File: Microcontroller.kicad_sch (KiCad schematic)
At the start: 33 parts, among them J501 USB4105-GF-A, J502 TC2030-CTX, SW501 PTS526SK15SMTR2 LFS, U501 USBLC6-2SC6, U502 STM32G441KBT6, Y501 ATS08A-E

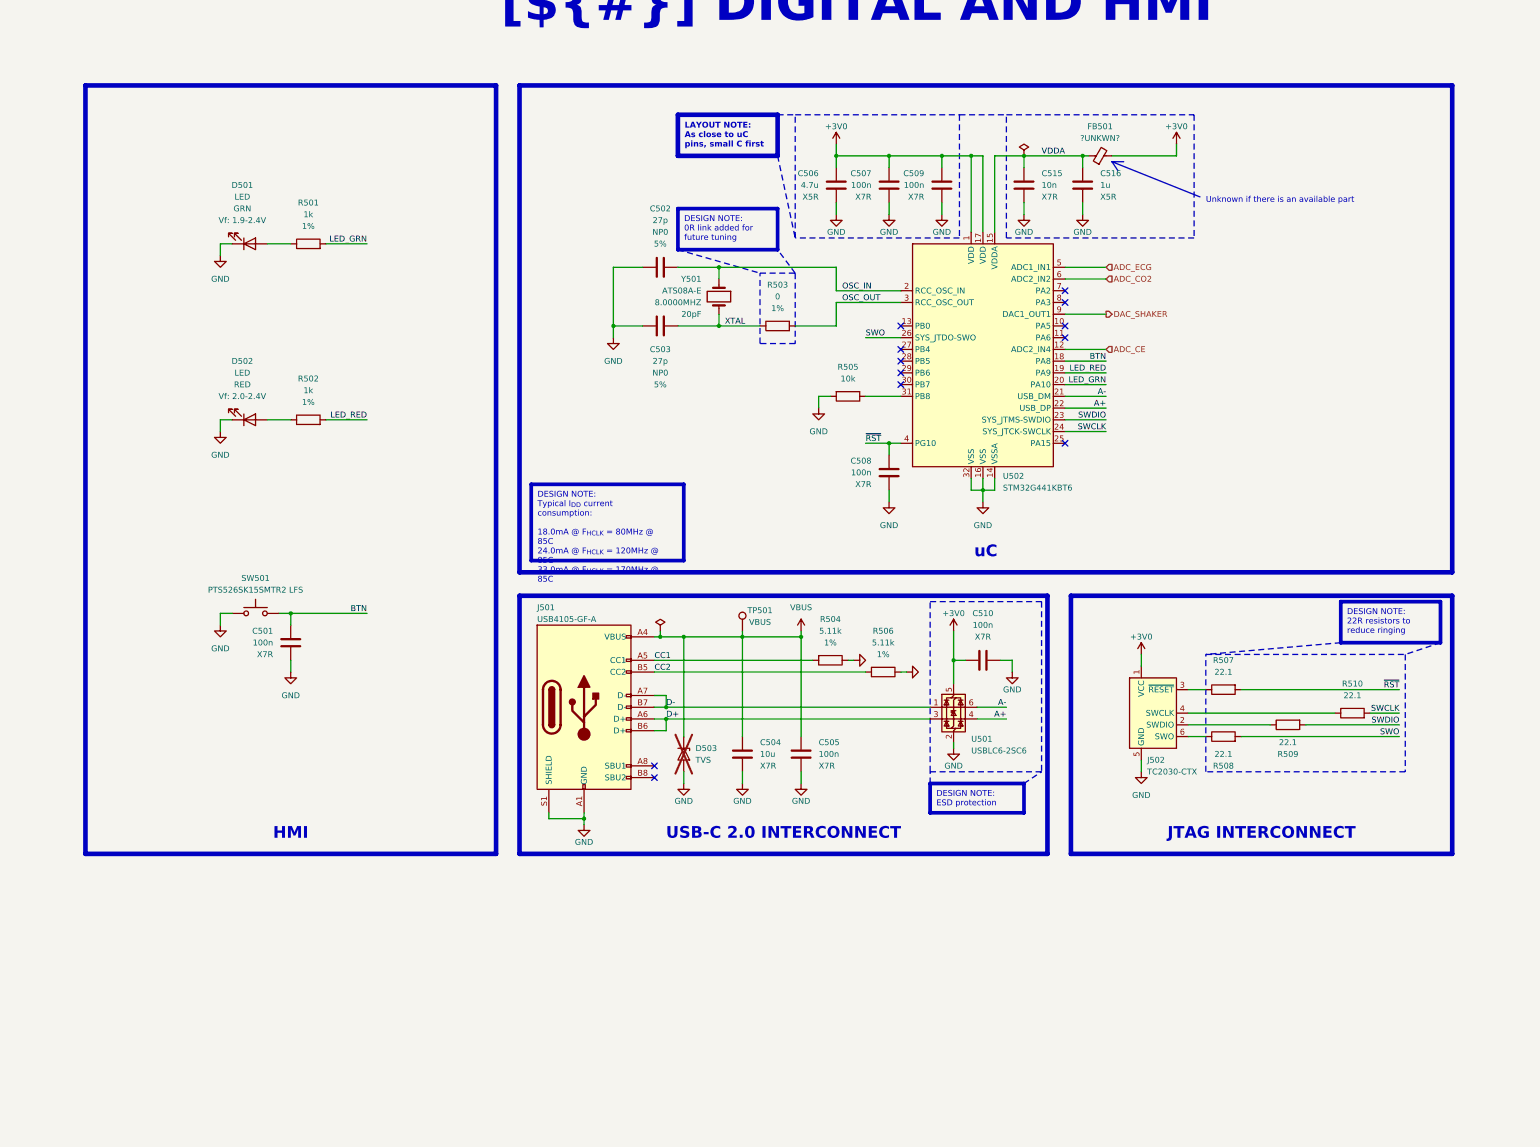
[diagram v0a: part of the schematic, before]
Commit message: feat: checked REV A
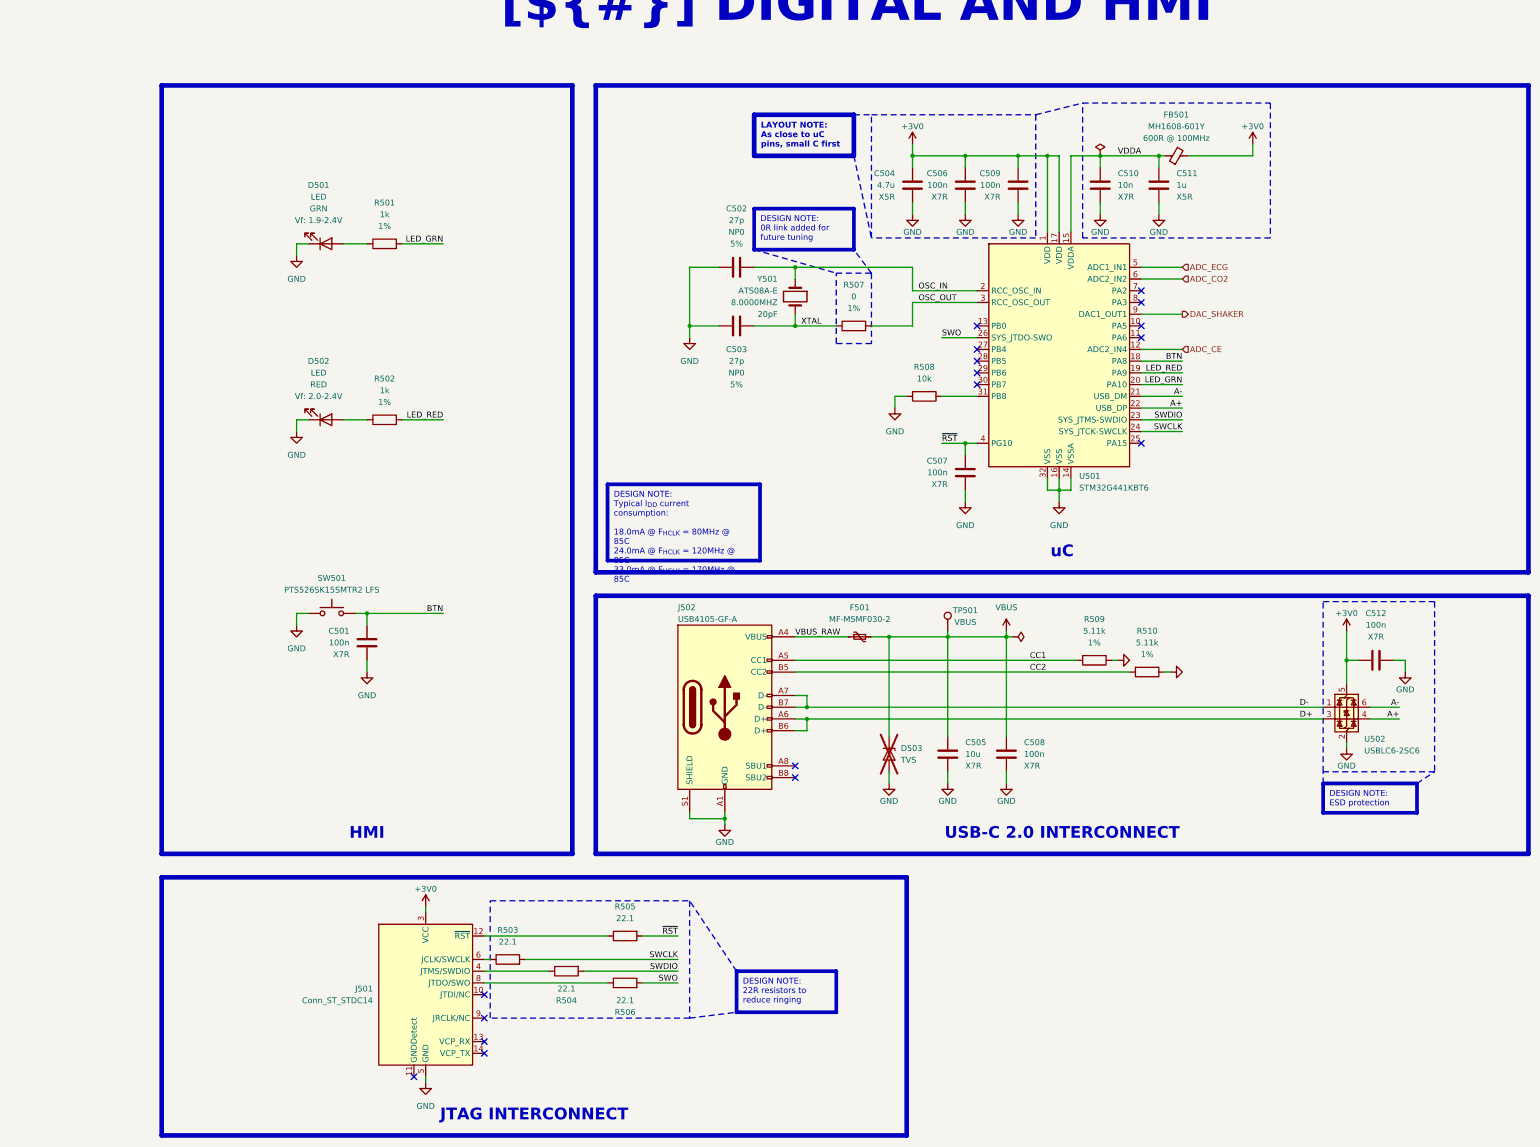
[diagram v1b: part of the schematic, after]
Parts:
- removed J502: TC2030-CTX, Connector:Tag-Connect_TC2030-IDC-NL_2x03_P1.27mm_Vertical, symbol Connector:Conn_ARM_SWD_TagConnect_TC2030-NL
- added F501: MF-MSMF030-2, Resistor_SMD:R_1812_4532Metric, symbol Device:Polyfuse_Small
- added J501: Conn_ST_STDC14, Connector_PinHeader_1.27mm:PinHeader_2x07_P1.27mm_Vertical_SMD, symbol Connector:Conn_ST_STDC14
- FB501: value ?UNKWN? -> MH1608-601Y; footprint (none) -> Inductor_SMD:L_0603_1608Metric; Impedance (none) -> 600R @ 100MHz; MPN (none) -> MH1608-601Y; Manufacturer (none) -> Bourns Inc.; SPN (none) -> MH1608-601YCT-ND; Supplier (none) -> DigiKey
- renumbered C506 to C504, C504 to C505, C507 to C506, C508 to C507, C505 to C508, C515 to C510, C516 to C511, C510 to C512, J501 to J502, R510 to R503, R509 to R504, R507 to R505, R508 to R506, R503 to R507, R505 to R508, R504 to R509, R506 to R510, U502 to U501, U501 to U502
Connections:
- net +3V0: now also J501.3 (VCC)
- net GND: now also J501.5 (GND), J501.7 (GND)
- net VBUS: now also F501.2; no longer J502.A4 (VBUS), J502.A9 (VBUS), J502.B4 (VBUS), J502.B9 (VBUS)
- net at R504.1: now also J501.4 (JTMS/SWDIO)
- net at R505.1: now also J501.12 (~{RST})
- net at R503.1: now also J501.6 (JCLK/SWCLK)
- net at R506.1: now also J501.8 (JTDO/SWO)
- new net VBUS_RAW: F501.1, J502.A4 (VBUS), J502.A9 (VBUS), J502.B4 (VBUS), J502.B9 (VBUS)
- no-connect marks 12 -> 17
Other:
- note removed: "Unknown if there is an available part"
- moved on the sheet: C501, C502, C503, C504, C505, C506, C507, C508, C509, C510, C511, C512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
